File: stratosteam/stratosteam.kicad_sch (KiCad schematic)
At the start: 7 parts, among them U1 RA-02_LORA, U2 NEO-M8M-0, U3 INA219AID, U4 BME280, U5 MS5611-01BA03, U6 BNO085, U7 AD9833

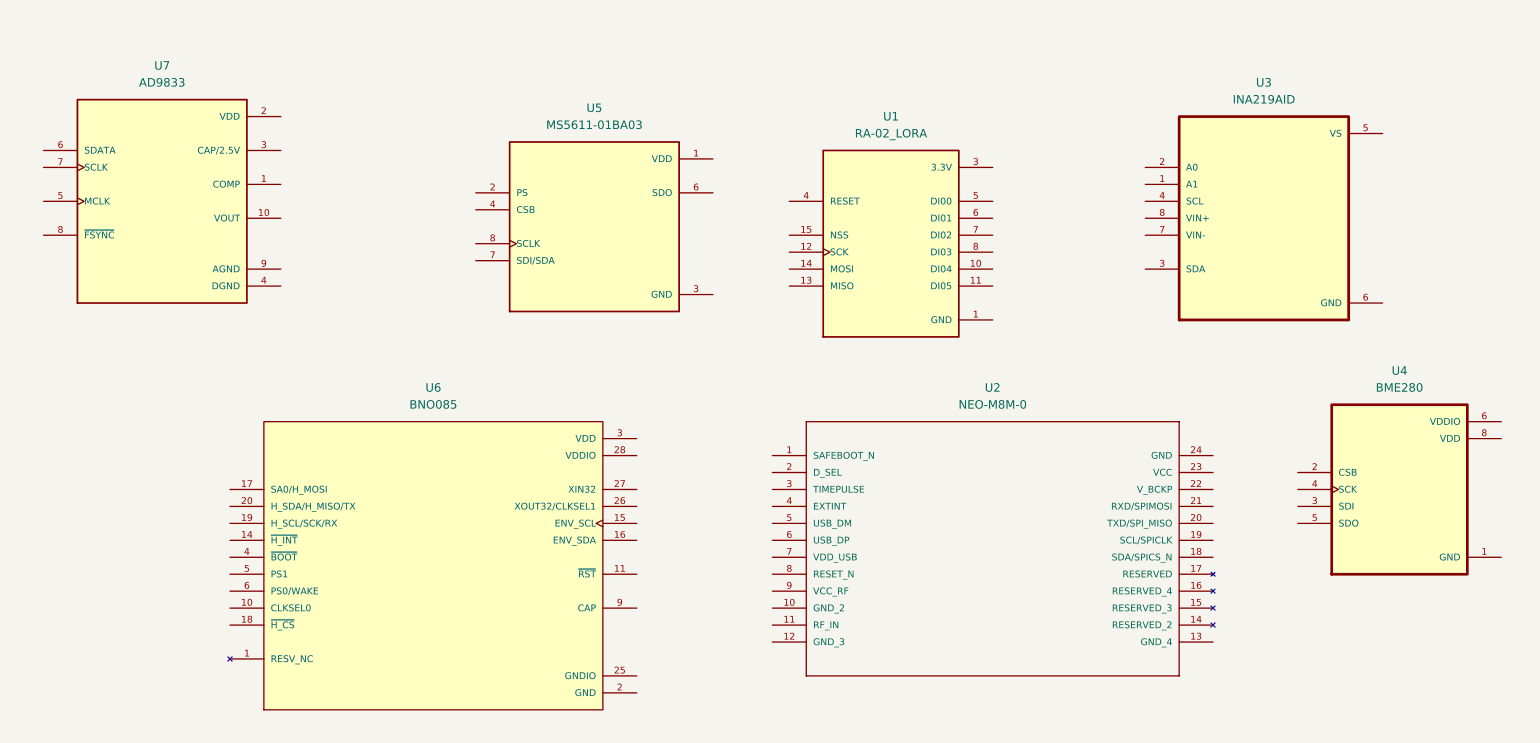
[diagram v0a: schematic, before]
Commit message: pcb
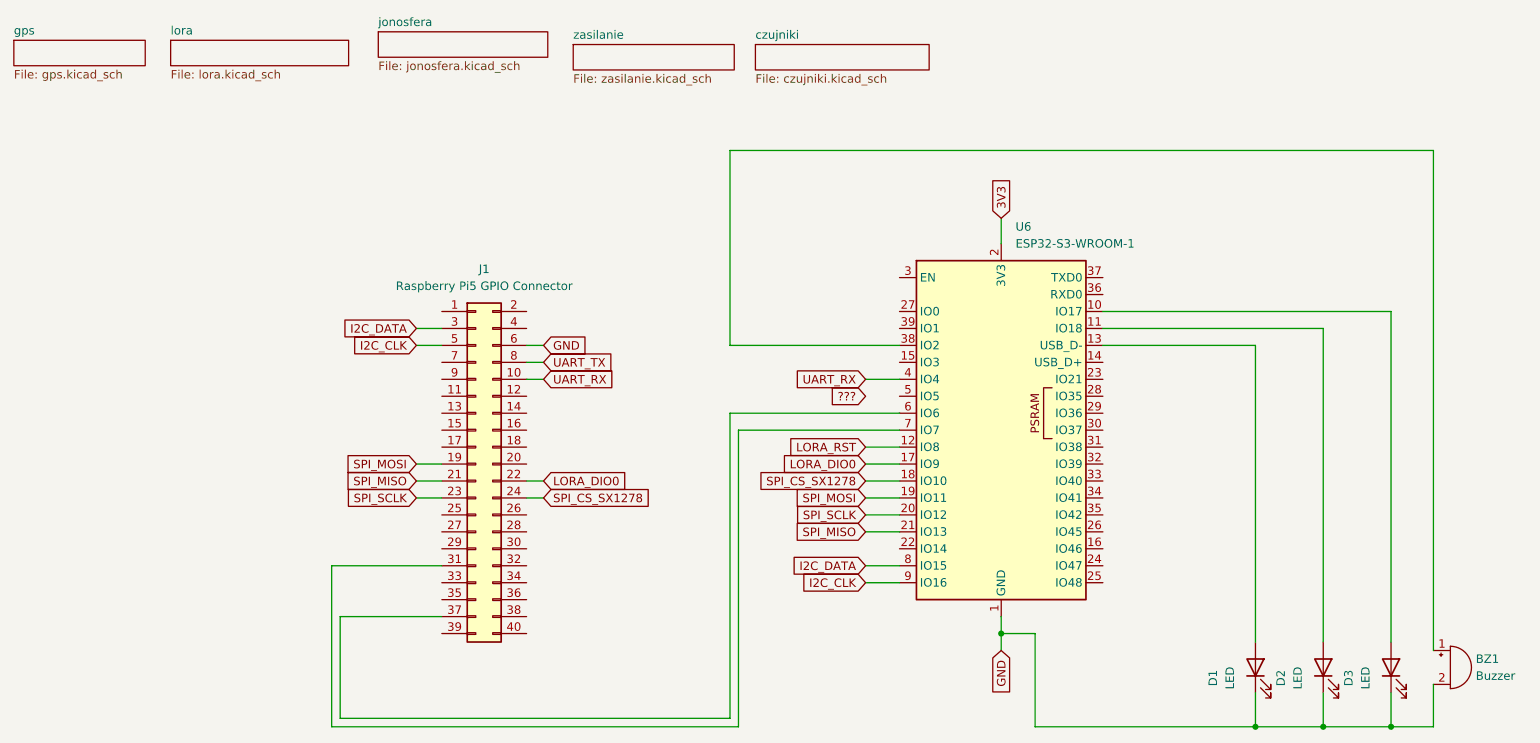
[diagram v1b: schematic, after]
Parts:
- removed U1: RA-02_LORA, RA-02_LORA:MODULE_RA-02_LORA, symbol RA-02_LORA:RA-02_LORA
- removed U2: NEO-M8M-0, NEO-M8M-0:NEO-M8_UBL, symbol NEO-M8M-0:NEO-M8M-0
- removed U3: INA219AID, INA219AID:SOIC127P599X175-8N, symbol INA219AID:INA219AID
- removed U4: BME280, BME280:PSON65P250X250X100-8N, symbol BME280:BME280
- removed U5: MS5611-01BA03, MS5611-01BA03:SON125P500X300X100-8N, symbol MS5611-01BA03:MS5611-01BA03
- removed U6: BNO085, BNO085:IC_BNO085, symbol BNO085:BNO085
- removed U7: AD9833, AD9833:SOP50P490X110-10N, symbol AD9833:AD9833
- added BZ1: Buzzer, Buzzer_Beeper:Buzzer_12x9.5RM7.6, symbol Device:Buzzer
- added D1, D2, D3: LED, LED_THT:LED_D3.0mm, symbol Device:LED
- added J1: Raspberry Pi5 GPIO Connector, symbol Connector_Generic:Conn_02x20_Odd_Even
- added U6: ESP32-S3-WROOM-1, RF_Module:ESP32-S3-WROOM-1, symbol RF_Module:ESP32-S3-WROOM-1
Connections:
- net GND: now also BZ1.2 (-), D1.1 (K), D2.1 (K), D3.1 (K), J1.6 (Pin_6), U6.1 (GND), U6.40 (GND), U6.41 (GND)
- new net: D2.2 (A), U6.11 (IO18)
- new net: BZ1.1 (+), U6.38 (IO2)
- new net: D3.2 (A), U6.10 (IO17)
- new net: J1.31 (Pin_31), U6.7 (IO7)
- new net: J1.37 (Pin_37), U6.6 (IO6)
- new net: D1.2 (A), U6.13 (USB_D-)
- new net 3V3: U6.2 (3V3)
- new net I2C_CLK: J1.5 (Pin_5), U6.9 (IO16)
- new net I2C_DATA: J1.3 (Pin_3), U6.8 (IO15)
- new net LORA_DIO0: J1.22 (Pin_22), U6.17 (IO9)
- new net LORA_RST: U6.12 (IO8)
- new net SPI_CS_SX1278: J1.24 (Pin_24), U6.18 (IO10)
- new net SPI_MISO: J1.21 (Pin_21), U6.21 (IO13)
- new net SPI_MOSI: J1.19 (Pin_19), U6.19 (IO11)
- new net SPI_SCLK: J1.23 (Pin_23), U6.20 (IO12)
- new net UART_RX: J1.10 (Pin_10), U6.4 (IO4)
- new net UART_TX: J1.8 (Pin_8)
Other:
- added sheet czujniki (czujniki.kicad_sch)
- added sheet gps (gps.kicad_sch)
- added sheet jonosfera (jonosfera.kicad_sch)
- added sheet lora (lora.kicad_sch)
- added sheet zasilanie (zasilanie.kicad_sch)
